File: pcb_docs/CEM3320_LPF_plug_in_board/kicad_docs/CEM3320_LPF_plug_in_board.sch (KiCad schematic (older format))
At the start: 42 parts, among them J1 signal_in, J2 signal_in, J3 signal_out, J4 Conn_01x08_Male, U1 CEM3320, U2 TL072

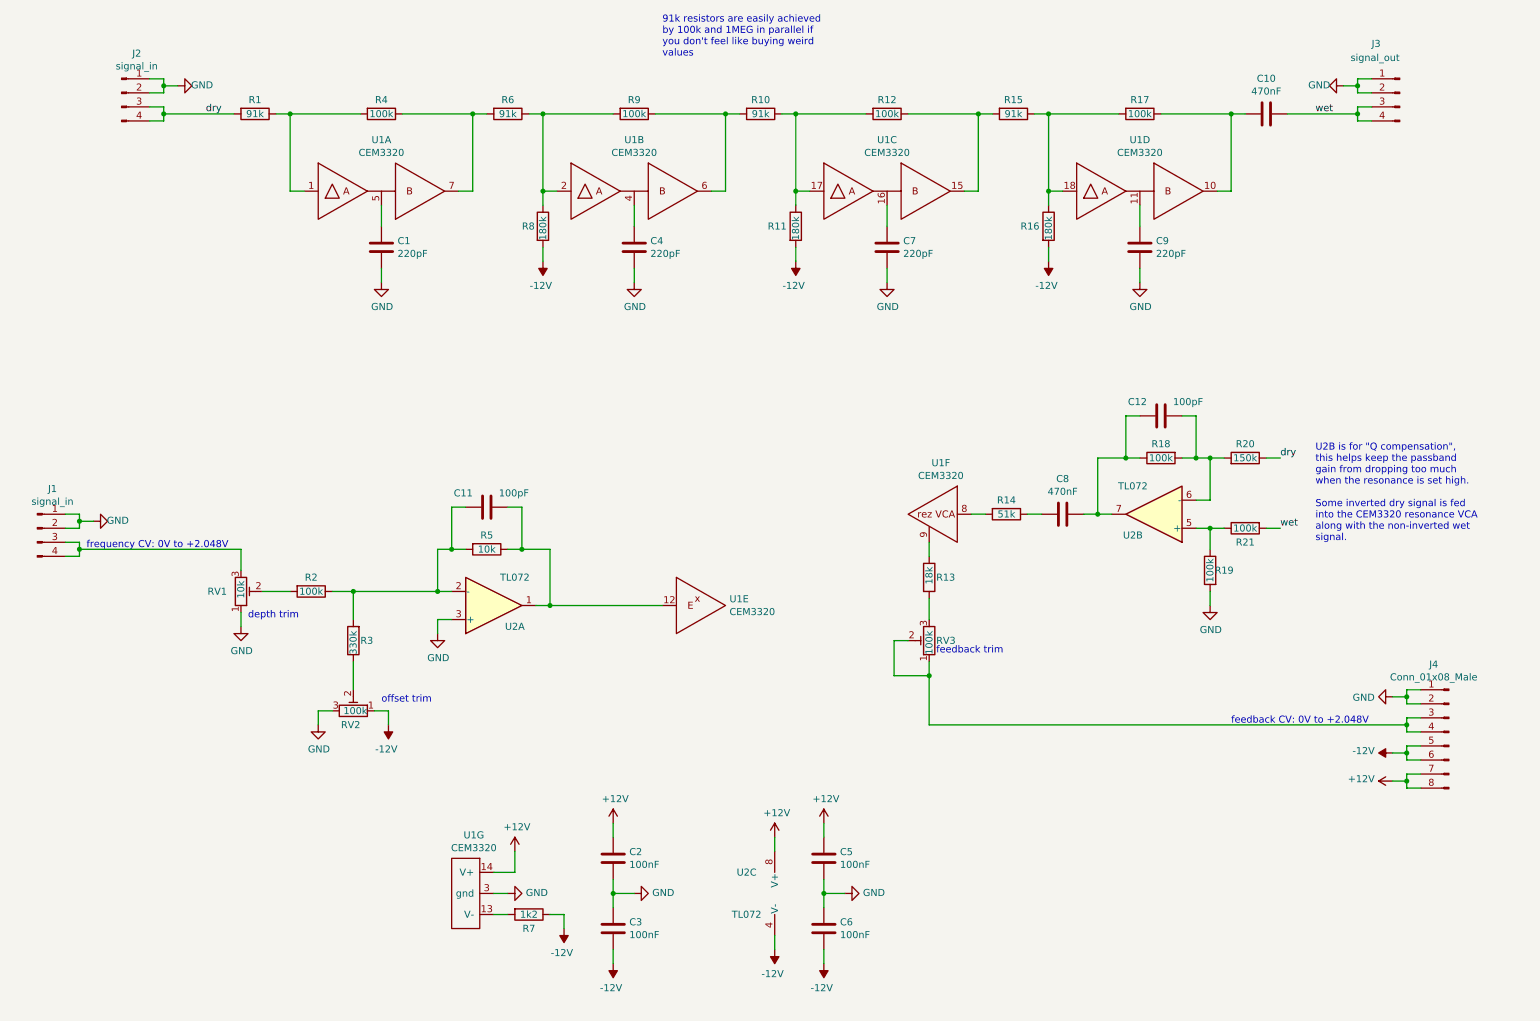
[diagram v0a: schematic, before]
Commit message: update CEM3320 VCF
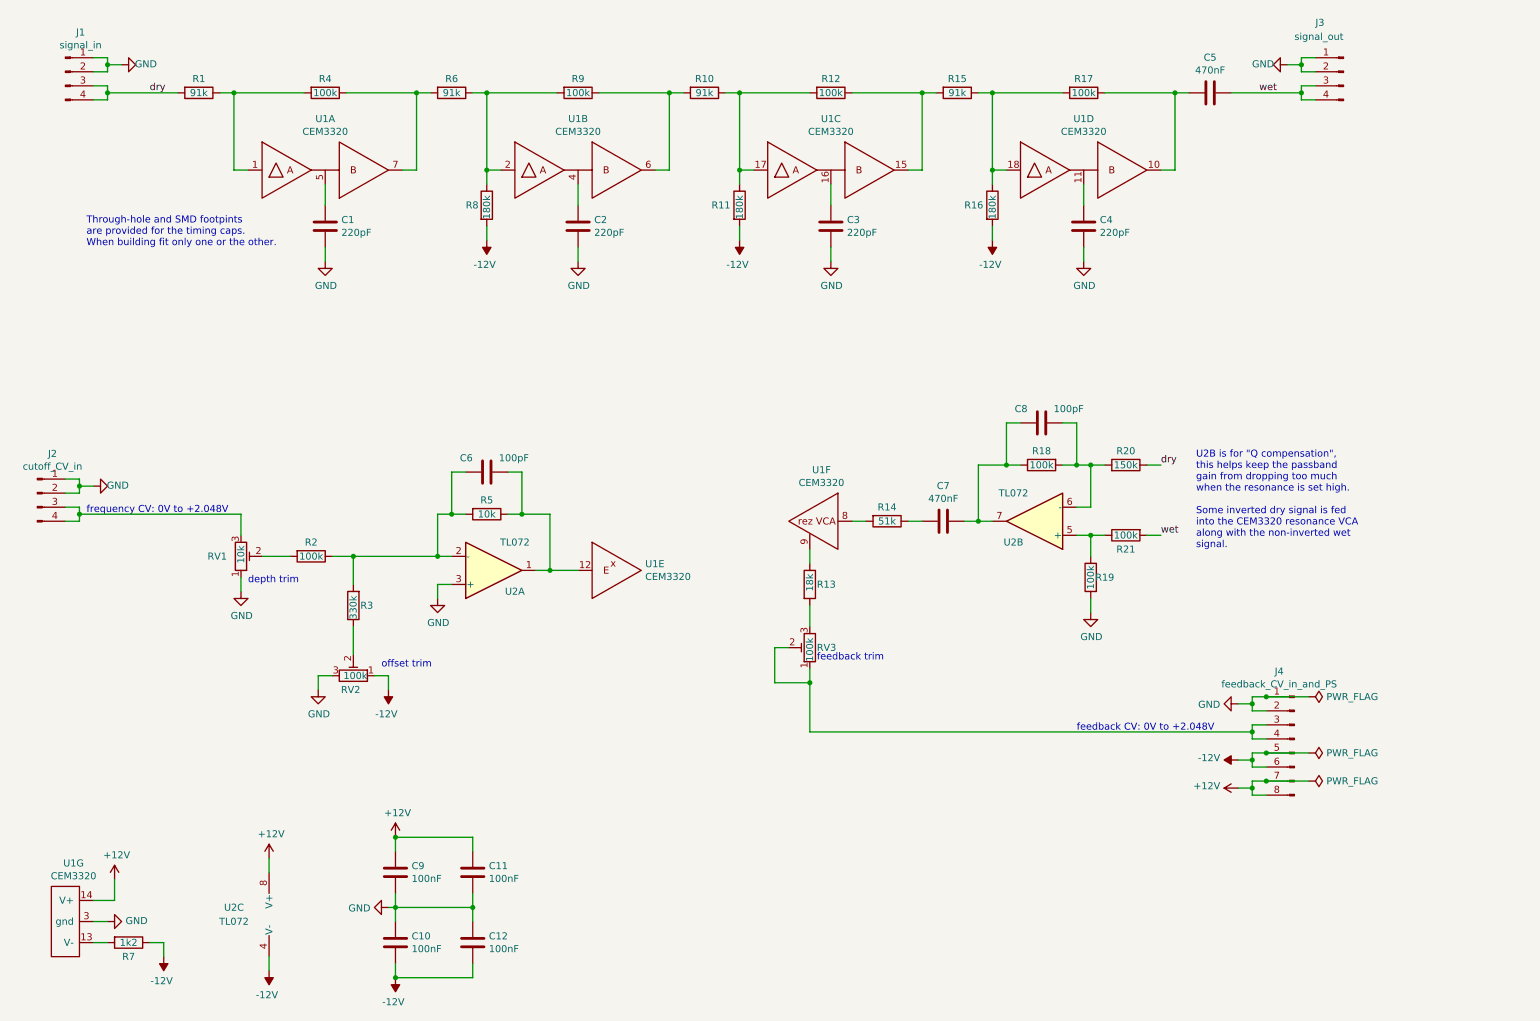
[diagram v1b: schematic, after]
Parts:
- removed C7, C9: 220pF, Capacitor_THT:C_Rect_L7.0mm_W4.5mm_P5.00mm, symbol Device:C
- added C2, C3: 220pF, cem3320:timing_cap_dual_fp, symbol Device:C
- C1, C4: footprint Capacitor_THT:C_Rect_L7.0mm_W4.5mm_P5.00mm -> cem3320:timing_cap_dual_fp
- J2: renamed from J1; value signal_in -> cutoff_CV_in
- J4: value Conn_01x08_Male -> feedback_CV_in_and_PS
- renumbered C3 to C10, C5 to C11, C6 to C12, C10 to C5, C11 to C6, C8 to C7, C12 to C8, C2 to C9, J2 to J1
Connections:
- net GND: now also C2.2, C3.2
- net at U1.4: now also C2.1; no longer C4.1
- net at U1.16: now also C3.1
- net at U1.11: now also C4.1
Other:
- note added: "Through-hole and SMD footpints\nare provided for the timing caps.\nWhen building fit only one or the other."
- note removed: "91k resistors are easily achieved \nby 100k and 1MEG in parallel if\nyou don't feel like buying weird \nvalues"
- moved on the sheet: C1, C10, C11, C12, C5, C6, C7, C8, C9, J1, J2, J3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
